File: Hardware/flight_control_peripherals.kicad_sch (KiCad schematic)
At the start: 16 parts, among them J11 Conn_02x06_Odd_Even, J12 Conn_01x06, J14 Micro_SD_Card_Det1, J6 Conn_01x10, J7 Conn_02x10_Odd_Even, J8 Conn_01x04, J9 Conn_01x04, U13 W25N01GVZEIG_TR, U14 24CW1280T-I/OT, U15 PCA9685PW_118

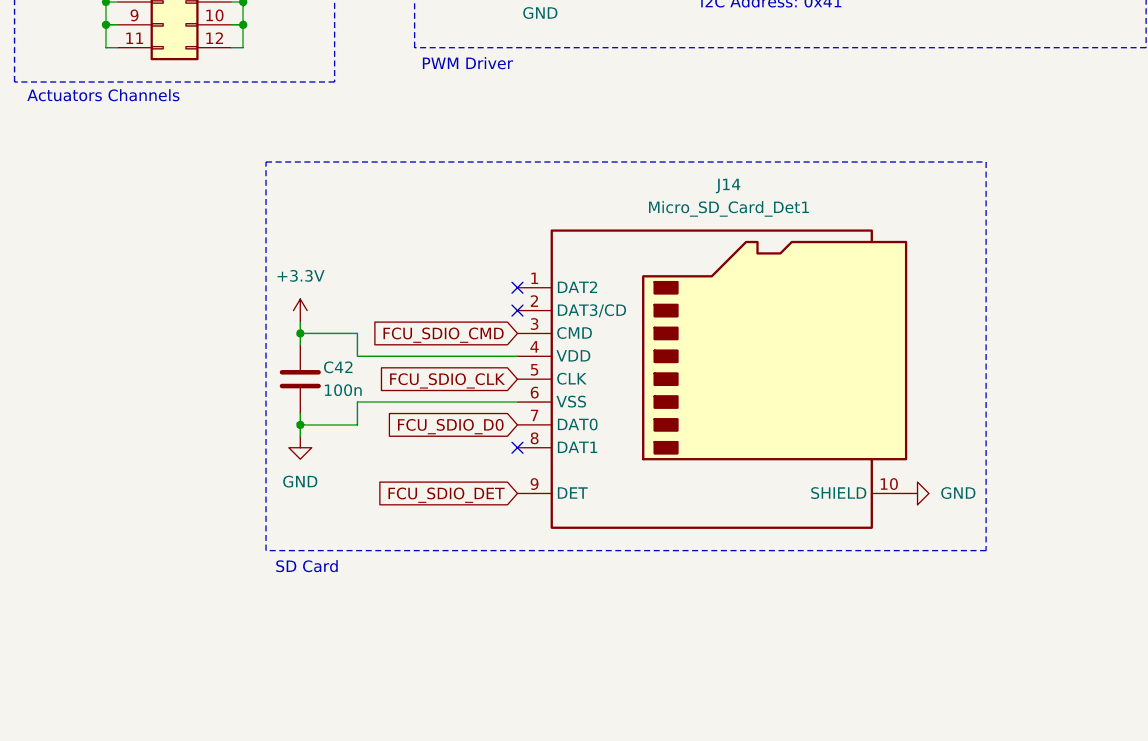
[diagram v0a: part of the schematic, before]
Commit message: sd card receptacle 10u capacitor
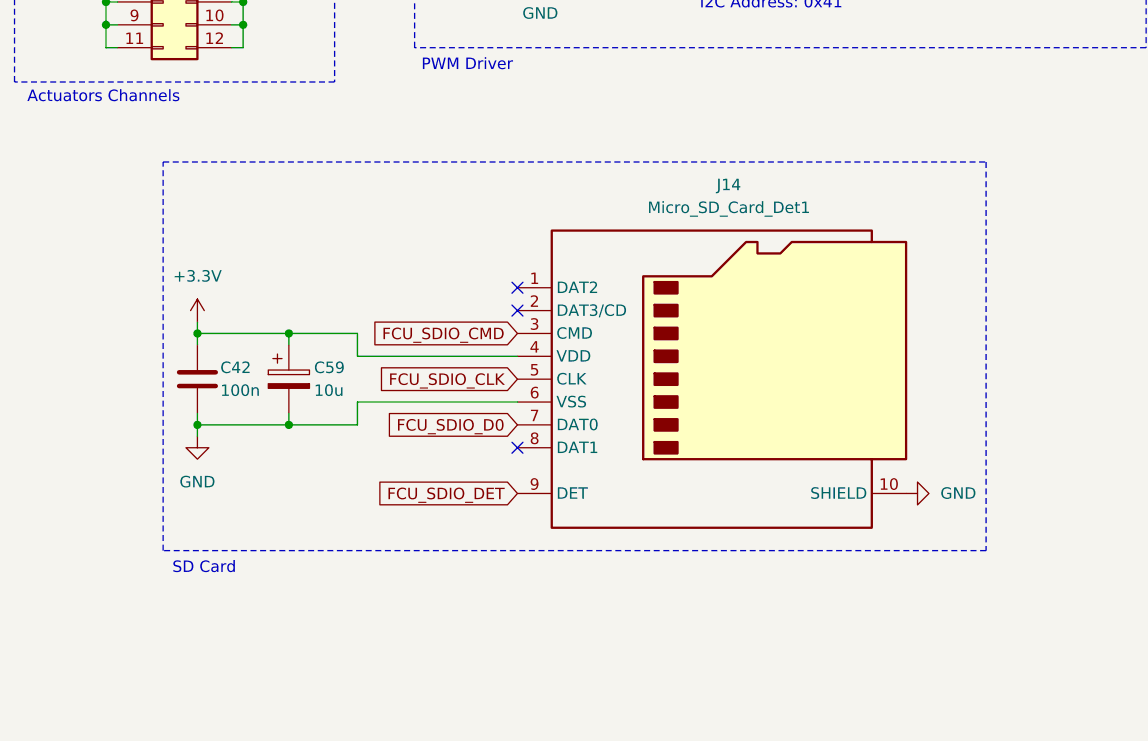
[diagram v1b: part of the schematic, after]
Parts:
- added C59: 10u, symbol Device:C_Polarized
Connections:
- net +3.3V: now also C59.1
- net GND: now also C59.2
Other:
- moved on the sheet: C42
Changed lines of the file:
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@@
 	)
 	(rectangle
-		(start 179.07 100.33)
+		(start 167.64 100.33)
 		(end 259.08 143.51)
 		(stroke
@@
 	(text "SD Card"
 		(exclude_from_sim no)
-		(at 183.642 145.542 0)
+		(at 172.212 145.542 0)
 		(effects
 			(font
@@
 	)
 	(junction
-		(at 182.88 119.38)
+		(at 171.45 119.38)
 		(diameter 0)
 		(color 0 0 0 0)
@@
 	)
 	(junction
-		(at 182.88 129.54)
+		(at 171.45 129.54)
 		(diameter 0)
 		(color 0 0 0 0)
@@
 	)
 	(junction
+		(at 181.61 119.38)
+		(diameter 0)
+		(color 0 0 0 0)
+	)
+	(junction
 		(at 209.55 74.93)
 		(diameter 0)
@@
 	)
 	(junction
+		(at 181.61 129.54)
+		(diameter 0)
+		(color 0 0 0 0)
+	)
+	(junction
 		(at 176.53 77.47)
 		(diameter 0)
@@
 	(wire
 		(pts
-			(xy 182.88 118.11) (xy 182.88 119.38)
+			(xy 171.45 118.11) (xy 171.45 119.38)
 		)
 		(stroke
@@
 	(wire
 		(pts
-			(xy 182.88 119.38) (xy 182.88 120.65)
+			(xy 171.45 119.38) (xy 171.45 120.65)
 		)
 		(stroke
@@
 	(wire
 		(pts
-			(xy 182.88 129.54) (xy 182.88 130.81)
+			(xy 171.45 129.54) (xy 171.45 130.81)
 		)
 		(stroke
@@
 	(wire
 		(pts
-			(xy 182.88 129.54) (xy 189.23 129.54)
+			(xy 171.45 129.54) (xy 181.61 129.54)
 		)
 		(stroke
@@
 	(wire
 		(pts
+			(xy 181.61 119.38) (xy 189.23 119.38)
+		)
+		(stroke
+			(width 0)
+			(type default)
+		)
+	)
+	(wire
+		(pts
 			(xy 213.36 29.21) (xy 259.08 29.21)
 		)
@@
 	(wire
 		(pts
+			(xy 181.61 128.27) (xy 181.61 129.54)
+		)
+		(stroke
+			(width 0)
+			(type default)
+		)
+	)
+	(wire
+		(pts
 			(xy 176.53 77.47) (xy 175.26 77.47)
 		)
@@
 	(wire
 		(pts
+			(xy 181.61 129.54) (xy 189.23 129.54)
+		)
+		(stroke
+			(width 0)
+			(type default)
+		)
+	)
+	(wire
+		(pts
 			(xy 69.85 64.77) (xy 69.85 67.31)
 		)
@@
 	(wire
 		(pts
-			(xy 182.88 128.27) (xy 182.88 129.54)
+			(xy 171.45 128.27) (xy 171.45 129.54)
 		)
 		(stroke
@@
 	(wire
 		(pts
+			(xy 181.61 119.38) (xy 181.61 120.65)
+		)
+		(stroke
+			(width 0)
+			(type default)
+		)
+	)
+	(wire
+		(pts
 			(xy 209.55 74.93) (xy 198.12 74.93)
 		)
@@
 	(wire
 		(pts
-			(xy 182.88 119.38) (xy 189.23 119.38)
+			(xy 171.45 119.38) (xy 181.61 119.38)
 		)
 		(stroke
@@
 	)
 	(symbol
+		(lib_id "Device:C_Polarized")
+		(at 181.61 124.46 0)
+		(unit 1)
+		(exclude_from_sim no)
+		(in_bom yes)
+		(on_board yes)
+		(dnp no)
+		(property "Reference" "C59"
+			(at 184.404 123.19 0)
+			(effects
+				(font
+					(size 1.27 1.27)
+				)
+				(justify left)
+			)
+		)
+		(property "Value" "10u"
+			(at 184.404 125.73 0)
+			(effects
+				(font
+					(size 1.27 1.27)
+				)
+				(justify left)
+			)
+		)
+		(property "Footprint" ""
+			(at 182.5752 128.27 0)
+			(effects
+				(font
+					(size 1.27 1.27)
+				)
+				(hide yes)
+			)
+		)
+		(property "Datasheet" "~"
+			(at 181.61 124.46 0)
+			(effects
+				(font
+					(size 1.27 1.27)
+				)
+				(hide yes)
+			)
+		)
+		(property "Description" "Polarized capacitor"
+			(at 181.61 124.46 0)
+			(effects
+				(font
+					(size 1.27 1.27)
+				)
+				(hide yes)
+			)
+		)
+		(pin "1"
+		)
+		(pin "2"
+		)
+		(instances
+			(project ""
+				(path "/8dc22ddc-eb0a-4b80-a714-26a959e826d2/2b3e482d-66cf-439d-9529-121b0ac868e2"
+					(reference "C59")
+					(unit 1)
+				)
+			)
+		)
+	)
+	(symbol
 		(lib_id "power:+3.3V")
-		(at 182.88 118.11 0)
+		(at 171.45 118.11 0)
 		(unit 1)
 		(exclude_from_sim no)
@@
 		(fields_autoplaced yes)
 		(property "Reference" "#PWR085"
-			(at 182.88 121.92 0)
+			(at 171.45 121.92 0)
 			(effects
 				(font
@@
 		)
 		(property "Value" "+3.3V"
-			(at 182.88 113.03 0)
+			(at 171.45 113.03 0)
 			(effects
 				(font
@@
 		)
 		(property "Footprint" ""
-			(at 182.88 118.11 0)
+			(at 171.45 118.11 0)
 			(effects
 				(font
@@
 		)
 		(property "Datasheet" ""
-			(at 182.88 118.11 0)
+			(at 171.45 118.11 0)
 			(effects
 				(font
@@
 		)
 		(property "Description" "Power symbol creates a global label with name \"+3.3V\""
-			(at 182.88 118.11 0)
+			(at 171.45 118.11 0)
 			(effects
 				(font
@@
 	(symbol
 		(lib_id "power:GND")
-		(at 182.88 130.81 0)
+		(at 171.45 130.81 0)
 		(unit 1)
 		(exclude_from_sim no)
@@
 		(fields_autoplaced yes)
 		(property "Reference" "#PWR086"
-			(at 182.88 137.16 0)
+			(at 171.45 137.16 0)
 			(effects
 				(font
@@
 		)
 		(property "Value" "GND"
-			(at 182.88 135.89 0)
+			(at 171.45 135.89 0)
 			(effects
 				(font
@@
 		)
 		(property "Footprint" ""
-			(at 182.88 130.81 0)
+			(at 171.45 130.81 0)
 			(effects
 				(font
@@
 		)
 		(property "Datasheet" ""
-			(at 182.88 130.81 0)
+			(at 171.45 130.81 0)
 			(effects
 				(font
@@
 		)
 		(property "Description" "Power symbol creates a global label with name \"GND\" , ground"
-			(at 182.88 130.81 0)
+			(at 171.45 130.81 0)
 			(effects
 				(font
@@
 	(symbol
 		(lib_id "Device:C")
-		(at 182.88 124.46 0)
+		(at 171.45 124.46 0)
 		(unit 1)
 		(exclude_from_sim no)
@@
 		(dnp no)
 		(property "Reference" "C42"
-			(at 185.42 123.19 0)
+			(at 173.99 123.19 0)
 			(effects
 				(font
@@
 		)
 		(property "Value" "100n"
-			(at 185.42 125.73 0)
+			(at 173.99 125.73 0)
 			(effects
 				(font
@@
 		)
 		(property "Footprint" ""
-			(at 183.8452 128.27 0)
+			(at 172.4152 128.27 0)
 			(effects
 				(font
@@
 		)
 		(property "Datasheet" "~"
-			(at 182.88 124.46 0)
+			(at 171.45 124.46 0)
 			(effects
 				(font
@@
 		)
 		(property "Description" "Unpolarized capacitor"
-			(at 182.88 124.46 0)
+			(at 171.45 124.46 0)
 			(effects
 				(font
